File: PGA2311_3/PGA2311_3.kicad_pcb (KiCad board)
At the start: 2 copper layers, 234 x 58 mm, 205 parts, among them J201 3, J202 3, J203 2, J204 2, J301 Conn_01x16, J302 1, J303 Conn_01x02, J304 4, J305 4, J401 1, J402 3, J403 1, Q301 BC817-40, SW301 SW_Push, SW302 Encoder PEC11R, U201 OPA1678IDR, U202 CD74HCT4052, U203 CD74HCT4052, U204 LM337LM, U205 PGA2311UA, U206 LM317LIDR, U207 UA78L05AIDR, U301 TPS60403DBV, U302 WH1602B, U303 SN74LVC8T245DW, U304 STM32G070KBT6, U305 TLV1117-50IDC, U306 LP2985-33DBV, U307 SN74LVC2G17DBV

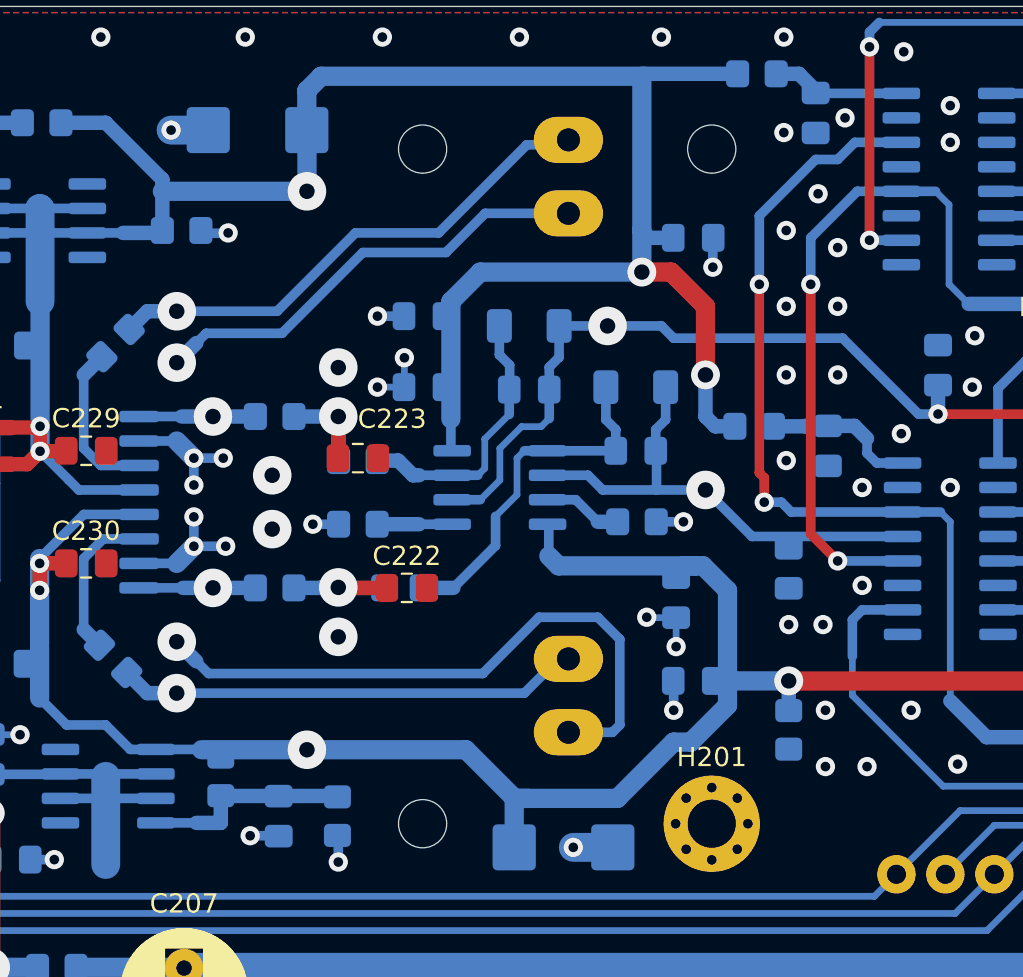
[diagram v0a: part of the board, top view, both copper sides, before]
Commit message: Add files via upload
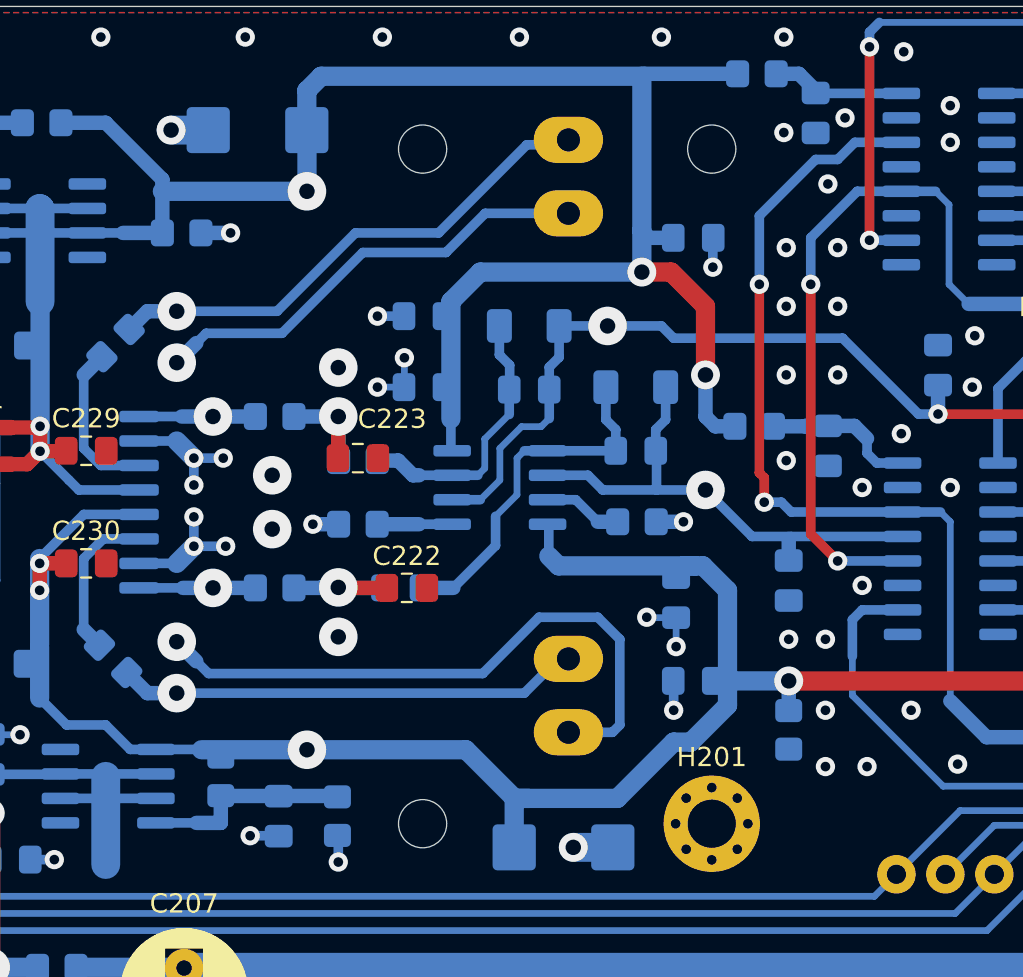
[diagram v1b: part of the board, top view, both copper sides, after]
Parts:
- moved C214 0.63 mm to (79.0, 49.8)
- moved R233 0.13 mm to (47.5, 31.8)
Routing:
- net Net-(U201A--): track 25.3 -> 26.6 mm
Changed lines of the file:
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@@
 	(footprint "Resistor_SMD:R_0805_2012Metric_Pad1.20x1.40mm_HandSolder"
 		(layer "B.Cu")
-		(at 47.498 31.623 180)
+		(at 47.498 31.75 180)
 		(descr "Resistor SMD 0805 (2012 Metric), square (rectangular) end terminal, IPC-7351 nominal with elongated pad for handsoldering. (Body size source: IPC-SM-782 page 72, https://www.pcb-3d.com/wordpress/wp-content/uploads/ipc-sm-782a_amendment_1_and_2.pdf), generated with kicad-footprint-generator")
 		(tags "resistor handsolder")
@@
 	(footprint "Capacitor_SMD:C_0805_2012Metric_Pad1.18x1.45mm_HandSolder"
 		(layer "B.Cu")
-		(at 78.994 49.149 -90)
+		(at 78.994 49.784 -90)
 		(descr "Capacitor SMD 0805 (2012 Metric), square (rectangular) end terminal, IPC-7351 nominal with elongated pad for handsoldering. (Body size source: IPC-SM-782 page 76, https://www.pcb-3d.com/wordpress/wp-content/uploads/ipc-sm-782a_amendment_1_and_2.pdf, https://docs.google.com/spreadsheets/d/1BsfQQcO9C6DZCsRaXUlFlo91Tg2WpOkGARC1WS5S8t0/edit?usp=sharing), generated with kicad-footprint-generator")
 		(tags "capacitor handsolder")
@@
 	)
 	(via
-		(at 80.772 52.07)
+		(at 80.899 52.832)
 		(size 1)
 		(drill 0.5)
@@
 	(via
 		(at 46.95062 26.416)
-		(size 1)
-		(drill 0.5)
+		(size 1.5)
+		(drill 0.8)
 		(layers "F.Cu" "B.Cu")
 		(free yes)
@@
 	)
 	(via
-		(at 49.911 31.75)
+		(at 50.038 31.75)
 		(size 1)
 		(drill 0.5)
@@
 	(via
 		(at 67.818 63.627)
-		(size 1)
-		(drill 0.5)
+		(size 1.5)
+		(drill 0.8)
 		(layers "F.Cu" "B.Cu")
 		(free yes)
@@
 	)
 	(via
-		(at 80.518 29.718)
+		(at 81.026 29.21)
 		(size 1)
 		(drill 0.5)
@@
 	)
 	(via
-		(at 78.994 52.07)
+		(at 78.994 52.832)
 		(size 1)
 		(drill 0.5)
@@
 	)
 	(via
-		(at 78.867 31.623)
+		(at 78.867 32.512)
 		(size 1)
 		(drill 0.5)
@@
 		(start 73.533 46.736)
 		(end 72.12 46.736)
-		(width 0.5)
+		(width 0.75)
 		(layer "B.Cu")
 		(net 1)
@@
 	)
 	(segment
-		(start 69.7405 63.627)
-		(end 69.8675 63.627)
-		(width 0.5)
+		(start 50.038 31.75)
+		(end 48.498 31.75)
+		(width 0.75)
 		(layer "B.Cu")
 		(net 1)
 	)
 	(segment
-		(start 49.895 31.766)
-		(end 48.514 31.766)
+		(start 69.7405 63.627)
+		(end 69.8675 63.627)
 		(width 0.5)
 		(layer "B.Cu")
@@
 	)
 	(segment
-		(start 48.498 31.75)
-		(end 48.498 31.623)
-		(width 0.5)
-		(layer "B.Cu")
-		(net 1)
-	)
-	(segment
 		(start 37.338 39.116)
 		(end 37.338 37.7405)
@@
 	)
 	(segment
-		(start 48.514 31.766)
-		(end 48.498 31.75)
-		(width 0.5)
-		(layer "B.Cu")
-		(net 1)
-	)
-	(segment
 		(start 47.244 52.959)
 		(end 48.26 53.975)
@@
 	)
 	(segment
-		(start 49.911 31.75)
-		(end 49.895 31.766)
-		(width 0.5)
-		(layer "B.Cu")
-		(net 1)
-	)
-	(segment
 		(start 75.057 33.528)
 		(end 75.057 32.0255)
@@
 		(start 54.3052 46.863)
 		(end 55.642 46.863)
-		(width 0.5)
+		(width 0.75)
 		(layer "B.Cu")
 		(net 1)
@@
 	)
 	(segment
+		(start 44.45 31.75)
+		(end 46.498 31.75)
+		(width 0.75)
+		(layer "B.Cu")
+		(net 2)
+	)
+	(segment
 		(start 71.374 33.782)
 		(end 71.374 31.623)
@@
 	)
 	(segment
-		(start 46.498 31.623)
-		(end 46.498 29.591)
-		(width 0.75)
-		(layer "B.Cu")
-		(net 2)
-	)
-	(segment
 		(start 76.2 41.783)
 		(end 75.184 41.783)
@@
 	)
 	(segment
-		(start 44.45 31.75)
-		(end 46.371 31.75)
-		(width 0.75)
-		(layer "B.Cu")
-		(net 2)
-	)
-	(segment
-		(start 46.371 31.75)
-		(end 46.498 31.623)
-		(width 0.75)
-		(layer "B.Cu")
-		(net 2)
-	)
-	(segment
 		(start 40.1535 31.623)
 		(end 40.1535 35.306)
@@
 	)
 	(segment
+		(start 46.498 31.75)
+		(end 46.498 29.591)
+		(width 0.75)
+		(layer "B.Cu")
+		(net 2)
+	)
+	(segment
 		(start 41.656 44.577)
 		(end 40.1535 43.0745)
@@
 	)
 	(segment
+		(start 78.994 48.7465)
+		(end 78.994 47.625)
+		(width 0.75)
+		(layer "B.Cu")
+		(net 101)
+	)
+	(segment
+		(start 78.994 47.625)
+		(end 79.121 47.498)
+		(width 0.25)
+		(layer "B.Cu")
+		(net 101)
+	)
+	(segment
 		(start 77.089 47.498)
-		(end 84.901 47.498)
+		(end 79.121 47.498)
 		(width 0.5)
 		(layer "B.Cu")
@@
 		(width 0.5)
 		(layer "B.Cu")
+		(net 101)
+	)
+	(segment
+		(start 79.121 47.498)
+		(end 84.901 47.498)
+		(width 0.5)
+		(layer "B.Cu")
